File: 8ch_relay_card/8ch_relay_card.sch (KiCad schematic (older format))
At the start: 19 parts

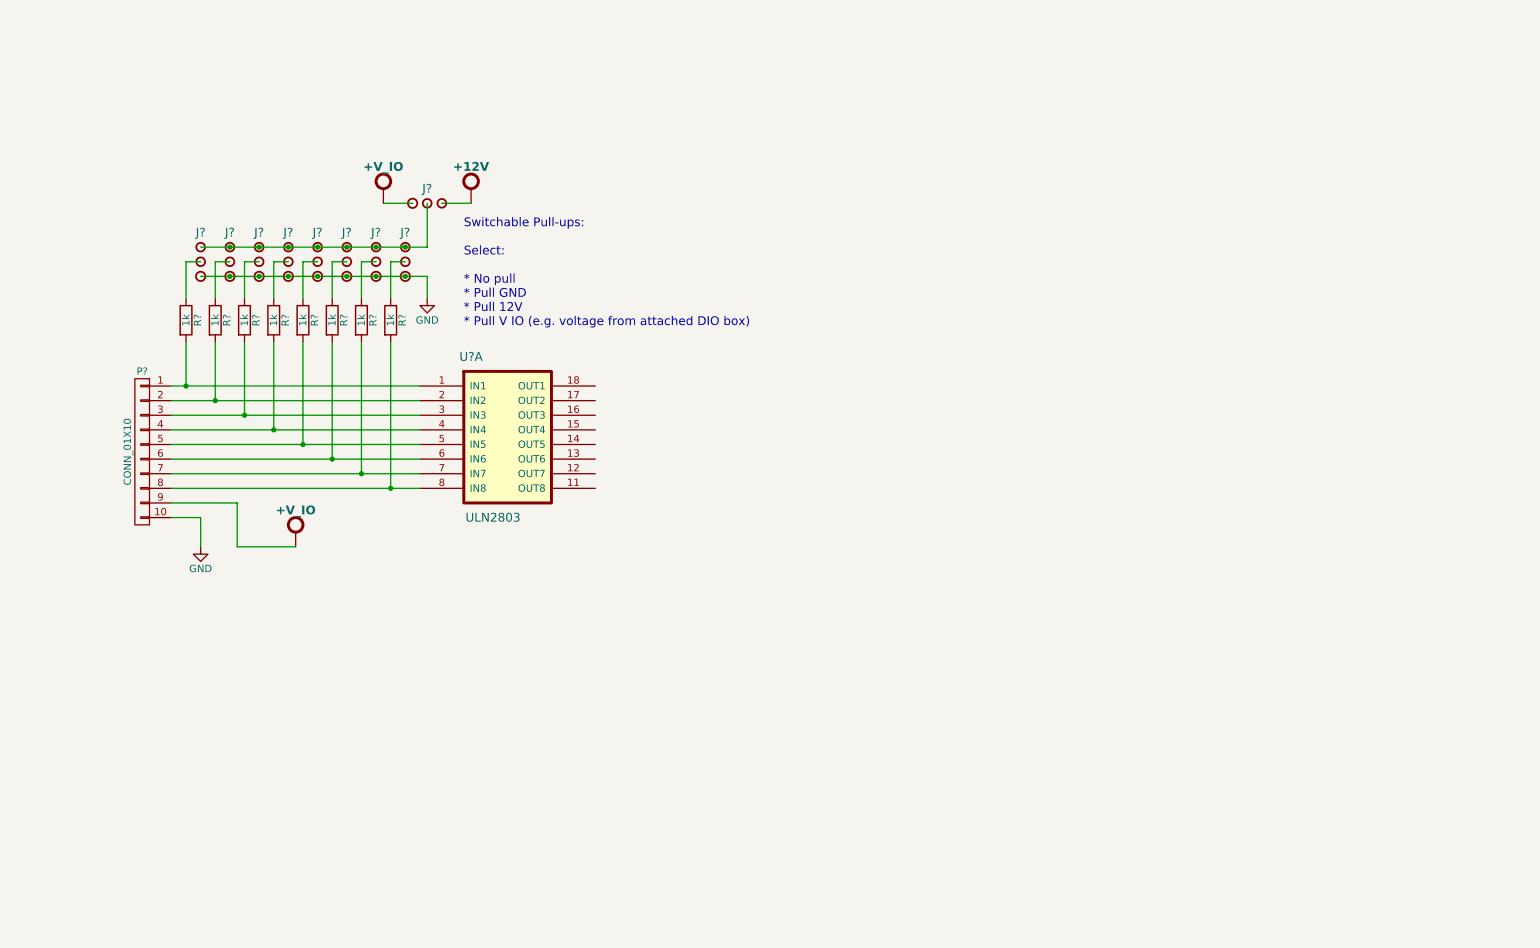
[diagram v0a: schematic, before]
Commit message: More work on the schematic
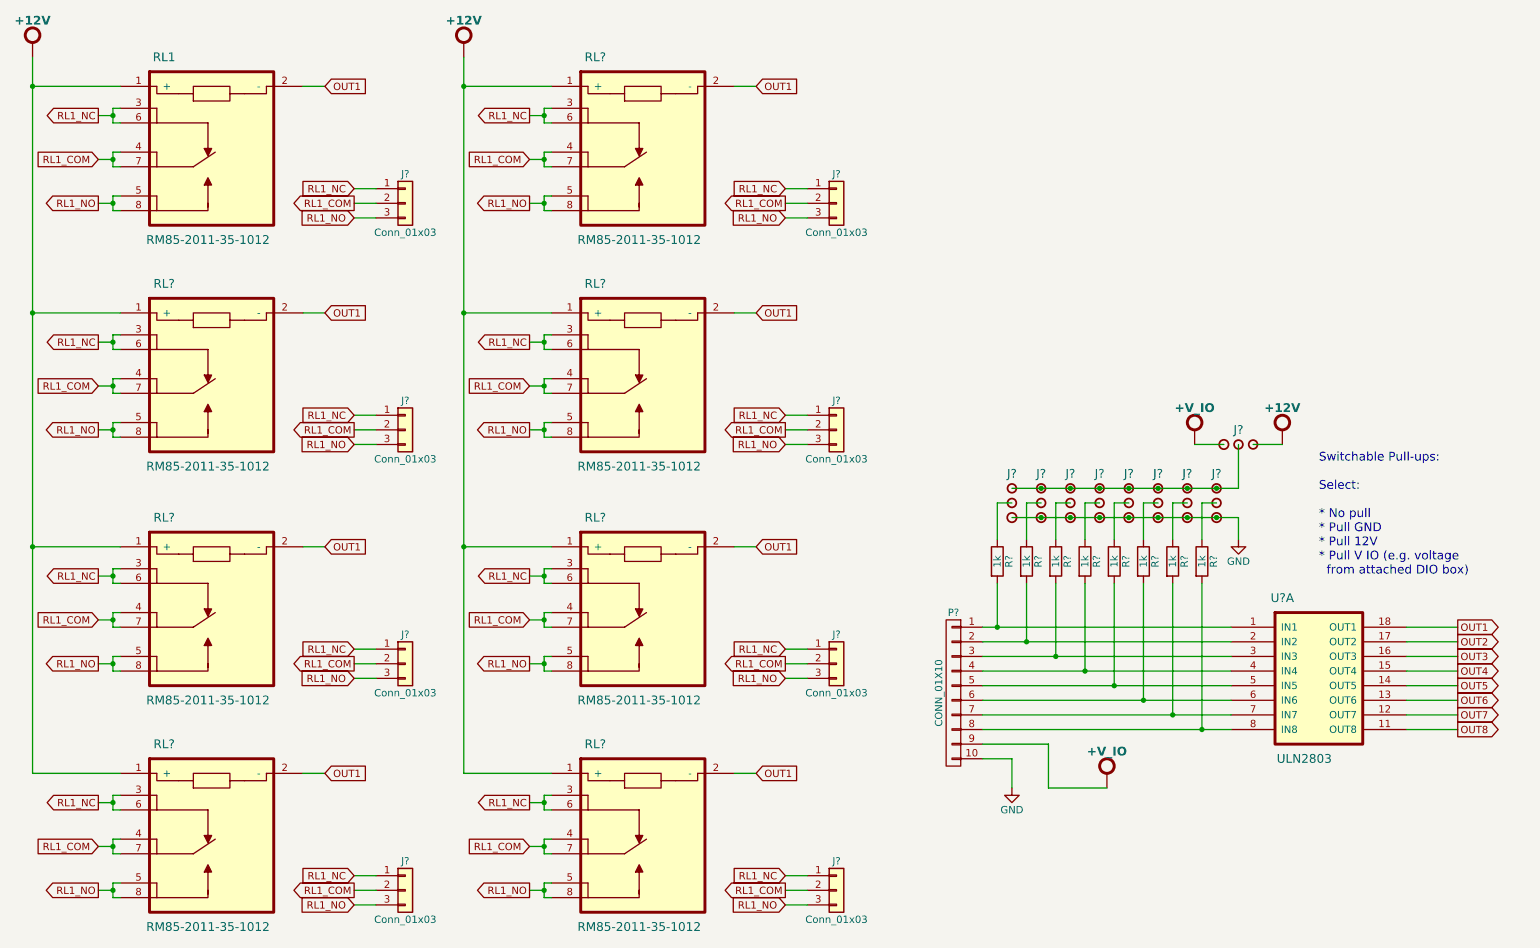
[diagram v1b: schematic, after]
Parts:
- added J? (x8): Conn_01x03, symbol Conn_01x03
- added RL1, RL? (x7): RM85-2011-35-1012, symbol RM85-2011-35-1012
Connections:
- net +12V: now also RL1.1 (+), RL?.1 (+), RL?.1 (+), RL?.1 (+), RL?.1 (+), RL?.1 (+), RL?.1 (+), RL?.1 (+)
- net OUT8: now reaches U?.11 (OUT8)
- net OUT7: now reaches U?.12 (OUT7)
- net OUT6: now reaches U?.13 (OUT6)
- net OUT5: now reaches U?.14 (OUT5)
- net OUT4: now reaches U?.15 (OUT4)
- net OUT3: now reaches U?.16 (OUT3)
- net OUT2: now reaches U?.17 (OUT2)
- net OUT1: now reaches U?.18 (OUT1)
- net OUT1: now also RL1.2 (-), RL?.2 (-), RL?.2 (-), RL?.2 (-), RL?.2 (-), RL?.2 (-), RL?.2 (-), RL?.2 (-)
- new net RL1_COM: J?.2 (Pin_2), J?.2 (Pin_2), J?.2 (Pin_2), J?.2 (Pin_2), J?.2 (Pin_2), J?.2 (Pin_2), J?.2 (Pin_2), J?.2 (Pin_2), RL1.4, RL1.7, RL?.4, RL?.4, RL?.4, RL?.4, RL?.4, RL?.4, RL?.4, RL?.7, RL?.7, RL?.7, RL?.7, RL?.7, RL?.7, RL?.7
- new net RL1_NC: J?.1 (Pin_1), J?.1 (Pin_1), J?.1 (Pin_1), J?.1 (Pin_1), J?.1 (Pin_1), J?.1 (Pin_1), J?.1 (Pin_1), J?.1 (Pin_1), RL1.3, RL1.6, RL?.3, RL?.3, RL?.3, RL?.3, RL?.3, RL?.3, RL?.3, RL?.6, RL?.6, RL?.6, RL?.6, RL?.6, RL?.6, RL?.6
- new net RL1_NO: J?.3 (Pin_3), J?.3 (Pin_3), J?.3 (Pin_3), J?.3 (Pin_3), J?.3 (Pin_3), J?.3 (Pin_3), J?.3 (Pin_3), J?.3 (Pin_3), RL1.5, RL1.8, RL?.5, RL?.5, RL?.5, RL?.5, RL?.5, RL?.5, RL?.5, RL?.8, RL?.8, RL?.8, RL?.8, RL?.8, RL?.8, RL?.8
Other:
- note added: "Switchable Pull-ups:\n\nSelect:\n\n* No pull\n* Pull GND\n* Pull 12V\n* Pull V IO (e.g. voltage \n from attached DIO box)"
- note removed: "Switchable Pull-ups:\n\nSelect:\n\n* No pull\n* Pull GND\n* Pull 12V\n* Pull V IO (e.g. voltage from attached DIO box)"
- moved on the sheet: J?, P?, R?, U?A
